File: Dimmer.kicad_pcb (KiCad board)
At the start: 2 copper layers, 63.9 x 63.9 mm, 21 parts, among them IC1 TTP224B-BSBN, J1 Reset, J2 Prog, J3 Conn_01x04, J4 Mode, J5 Load_cntrl, J6 Detect_null, U1 ESP-07, k1 Key, k2 Key, k3 Key

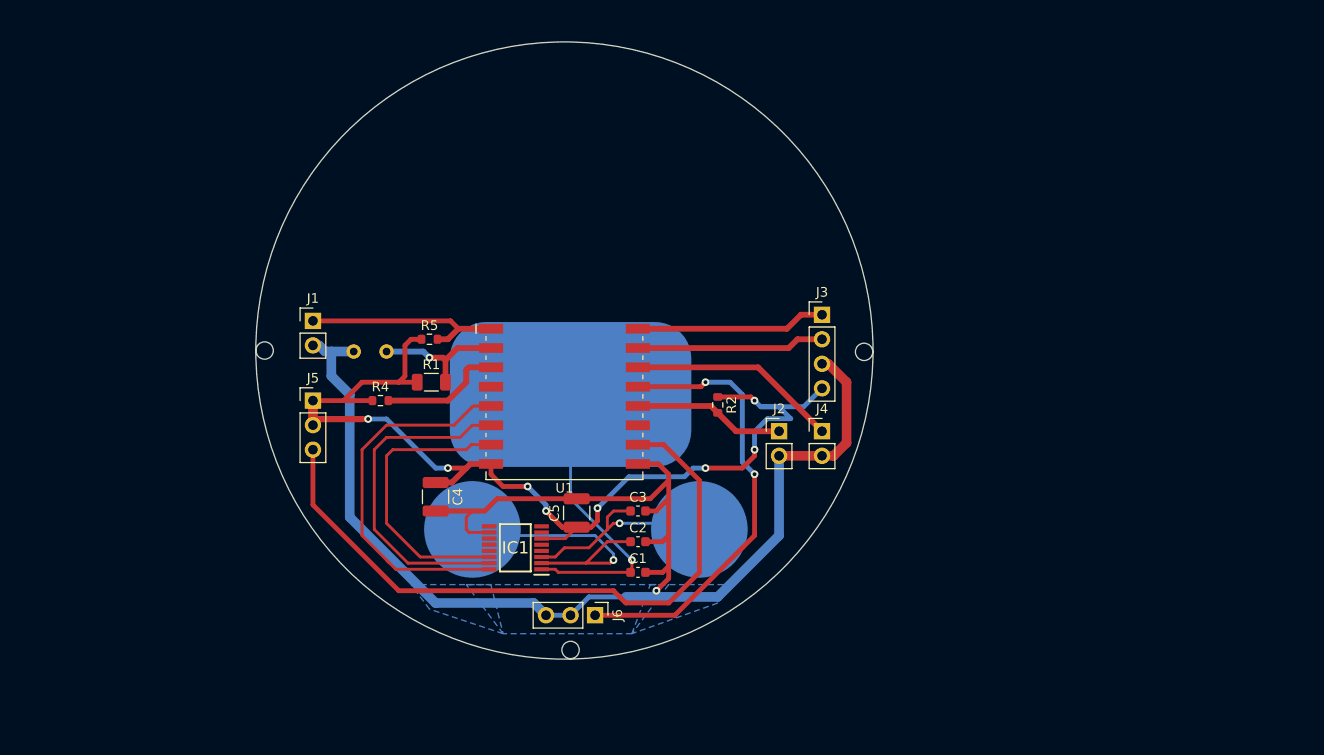
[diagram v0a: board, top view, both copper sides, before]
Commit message: Add files via upload
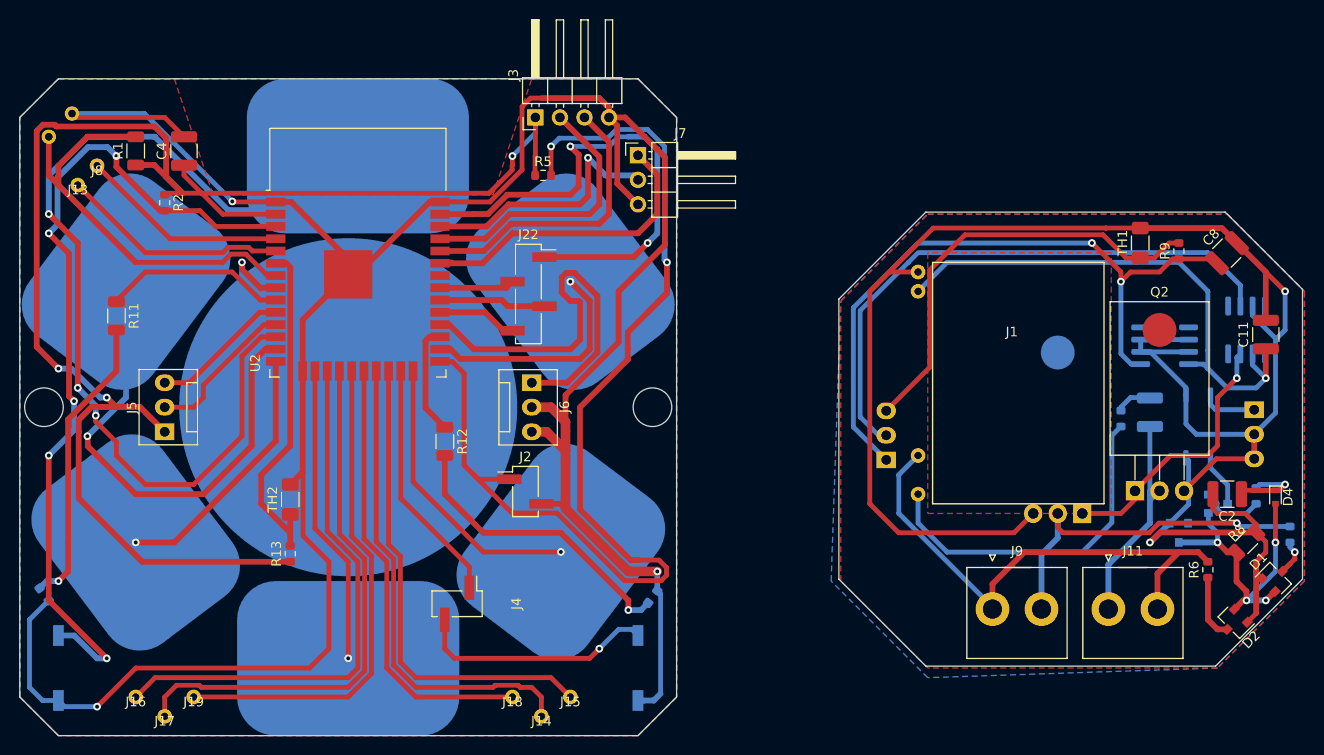
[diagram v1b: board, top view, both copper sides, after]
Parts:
- removed C3: 30p, Capacitor_SMD:C_0603_1608Metric
- removed C5: 100mk, Capacitor_SMD:C_1210_3225Metric
- removed IC1: TTP224B-BSBN, TTP224B-BSBN:SOP64P600X175-16N
- added C11: 0.33mk, Capacitor_SMD:C_1210_3225Metric, F.Cu at (232.0, 100.5)
- added C8: 0.1mk, Capacitor_SMD:C_1210_3225Metric, F.Cu at (228.0, 92.0)
- added D1: BAV99, Package_TO_SOT_SMD:SOT-23, F.Cu at (233.0, 125.7)
- added D2: BAV99, Package_TO_SOT_SMD:SOT-23, F.Cu at (228.7, 130.3)
- added D3: BZX84Cxx, Diode_SMD:D_SOT-23_ANK, B.Cu at (223.0, 121.0)
- added D4: 1N4148WT, Diode_SMD:D_SOD-523, F.Cu at (233.0, 117.3)
- added D5: BLUE, LED_SMD:LED_0603_1608Metric, B.Cu at (105.5, 127.4)
- added D6: RED, LED_SMD:LED_0603_1608Metric, B.Cu at (168.5, 127.6)
- added J10: Detect_nullA, Connector:FanPinHeader_1x03_P2.54mm_Vertical, B.Cu at (230.8, 108.3)
- added J11: 220v_OUT, Touch_pad:220V_1x02_P5.08mm_Horizontal, F.Cu at (215.7, 125.9)
- added J12: Load_cntrlA, Connector:FanPinHeader_1x03_P2.54mm_Vertical, B.Cu at (192.7, 113.5)
- added J13: ADC, Touch_pad:polz_razjem, F.Cu at (109.0, 85.0)
- added J14: Conn_01x01, Touch_pad:polz_razjem, F.Cu at (157.0, 140.0)
- added J15: Conn_01x01, Touch_pad:polz_razjem, F.Cu at (160.0, 138.0)
- added J16: Conn_01x01, Touch_pad:polz_razjem, F.Cu at (115.0, 138.0)
- added J17: Conn_01x01, Touch_pad:polz_razjem, F.Cu at (118.0, 140.0)
- added J18: Conn_01x01, Touch_pad:polz_razjem, F.Cu at (154.0, 138.0)
- added J19: Conn_01x01, Touch_pad:polz_razjem, F.Cu at (121.0, 138.0)
- added J22: SPI, Connector_PinHeader_2.54mm:PinHeader_1x04_P2.54mm_Vertical_SMD_Pin1Right, F.Cu at (155.7, 96.3)
- added J7: I2C, Connector_PinHeader_2.54mm:PinHeader_1x03_P2.54mm_Horizontal, F.Cu at (167.0, 81.9)
- added J8: ADC, Touch_pad:polz_razjem, F.Cu at (111.0, 83.0)
- added J9: 220v_IN, Touch_pad:220V_1x02_P5.08mm_Horizontal, F.Cu at (203.7, 125.9)
- added Q1: IRFP460APBF, Package_TO_SOT_THT:TO-220-3_Horizontal_TabDown, B.Cu at (213.0, 119.0)
- added Q2: IRFP460APBF, Package_TO_SOT_THT:TO-220-3_Horizontal_TabDown, F.Cu at (218.5, 116.7)
- added Q3: BC807, Package_TO_SOT_SMD:SOT-23, B.Cu at (227.1, 118.0)
- added R10: 220, Resistor_SMD:R_0603_1608Metric, B.Cu at (231.0, 117.2)
- added R11: 220, Resistor_SMD:R_1206_3216Metric, F.Cu at (113.0, 98.5)
- added R12: 220, Resistor_SMD:R_1206_3216Metric, F.Cu at (147.0, 111.5)
- added R13: 10k, Resistor_SMD:R_0603_1608Metric, F.Cu at (131.0, 123.2)
- added R6: 120k 0.25W, Resistor_SMD:R_0603_1608Metric, F.Cu at (226.0, 124.8)
- added R7: 220 1W, Resistor_SMD:R_0603_1608Metric, B.Cu at (217.0, 109.2)
- added R8: 330k 0.25W, Resistor_SMD:R_1206_3216Metric, F.Cu at (230.0, 122.0)
- added R9: 10k, Resistor_SMD:R_0603_1608Metric, F.Cu at (223.0, 91.8)
- added SW1: SW_Push, Button_Switch_SMD:SW_DIP_SPSTx01_Slide_6.7x4.1mm_W6.73mm_P2.54mm_LowProfile_JPin, B.Cu at (107.0, 135.0)
- added SW2: SW_Push, Button_Switch_SMD:SW_DIP_SPSTx01_Slide_6.7x4.1mm_W6.73mm_P2.54mm_LowProfile_JPin, B.Cu at (167.0, 135.0)
- added TH1: Thermistor_NTC, Resistor_SMD:R_1206_3216Metric_Pad1.30x1.75mm_HandSolder, F.Cu at (219.0, 91.0)
- added TH2: Thermistor_NTC, Resistor_SMD:R_1206_3216Metric_Pad1.30x1.75mm_HandSolder, F.Cu at (131.0, 117.5)
- added U2: ESP32-WROOM-32D, RF_Module:ESP32-WROOM-32, F.Cu at (138.0, 95.0)
- added U3: L78L33_SO8, Package_SO:SOIC-8_3.9x4.9mm_P1.27mm, B.Cu at (221.5, 101.6)
- added U4: TLP185, Package_SO:SOIC-4_4.55x3.7mm_P2.54mm, B.Cu at (225.0, 110.0)
- added k4: Key, Touch_pad:TestPoint_Pad_1.0x1.0sm, B.Cu at (107.0, 128.0)
- added k5: Key, Touch_pad:TestPoint_Pad_1.0x1.0sm, B.Cu at (137.0, 144.0)
- added k6: Key, Touch_pad:TestPoint_Pad_1.0x1.0sm, B.Cu at (122.0, 101.0)
- added k7: Key, Touch_pad:TestPoint_Pad_1.0x1.0sm, B.Cu at (138.0, 92.0)
- C1: value 30p -> 0.01mk; footprint Capacitor_SMD:C_0603_1608Metric -> Capacitor_SMD:C_1210_3225Metric; moved to B.Cu
- C2: value 30p -> 0.47mk; footprint Capacitor_SMD:C_0603_1608Metric -> Capacitor_SMD:C_1210_3225Metric
- J1: value Reset -> 220to12; footprint Connector_PinHeader_2.54mm:PinHeader_1x02_P2.54mm_Vertical -> Touch_pad:oblast_bp
- J2, J4: footprint Connector_PinHeader_2.54mm:PinHeader_1x02_P2.54mm_Vertical -> Connector_PinHeader_2.54mm:PinHeader_1x02_P2.54mm_Vertical_SMD_Pin1Left
- J3: value Conn_01x04 -> UART0; footprint Connector_PinHeader_2.54mm:PinHeader_1x04_P2.54mm_Vertical -> Connector_PinHeader_2.54mm:PinHeader_1x04_P2.54mm_Horizontal
- J5, J6: footprint Connector_PinHeader_2.54mm:PinHeader_1x03_P2.54mm_Vertical -> Connector:FanPinHeader_1x03_P2.54mm_Vertical
- R4: value 10k -> 120k 0.25W; moved to B.Cu
- U1: value ESP-07 -> FAN3268; footprint RF_Module:ESP-07 -> Package_SO:SOIC-8_3.9x4.9mm_P1.27mm; moved to B.Cu
- k1: footprint Touch_pad:TestPoint_Pad_2.5x2.5sm -> Touch_pad:TestPoint_Pad_1.0x1.0sm
- moved R4 95.2 mm to (234.5, 121.2), turned to 90 degrees
- moved J1 73.4 mm to (206.5, 105.0)
- moved U1 70.8 mm to (230.0, 100.0), turned to 270 degrees
- moved C2 61.2 mm to (228.0, 117.0), turned to 180 degrees
- moved R2 61.0 mm to (118.0, 86.8)
- moved C1 55.5 mm to (220.0, 108.5), turned to 270 degrees
- moved k3 46.4 mm to (137.0, 118.0), turned to 0 degrees
- moved C4 44.3 mm to (120.0, 81.5), turned to 90 degrees
- moved J4 41.8 mm to (148.3, 128.3), turned to 270 degrees
- moved R3 41.4 mm to (106.0, 80.0), turned to 45 degrees
- moved R1 38.9 mm to (115.0, 81.5), turned to 90 degrees
- moved J3 36.0 mm to (156.4, 78.0), turned to 90 degrees
- moved J2 27.0 mm to (155.3, 116.7)
- moved J6 25.0 mm to (156.0, 105.5)
- moved R5 20.6 mm to (157.2, 84.0)
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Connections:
- C1 pad 2: GND -> Net-(C1-Pad2)
- C2 pad 2: GND -> Net-(C2-Pad2)
- J1 pad 2: GND -> +12V
- J3 pad 1: Net-(J3-Pad1) -> +3V3
- J3 pad 3: GND -> Net-(J3-Pad3)
- J3 pad 4: +3V3 -> GND
- J4 pad 1: Net-(J4-Pad1) -> Mode
- J4 pad 2: GND -> Net-(J4-Pad2)
- J5 pad 2: +3V3 -> GPIO26
- J5 pad 3: GPIO15 -> GPIO32
- J6 pad 1: GPIO4 -> GPIO17
- R1 pad 2: Net-(R1-Pad2) -> GPIO35
- R2 pad 2: Net-(J2-Pad1) -> Net-(R2-Pad2)
- R3 pad 1: Net-(R1-Pad2) -> GPIO35
- R4 pad 1: +3V3 -> Net-(D1-Pad3)
- R4 pad 2: Net-(R4-Pad2) -> Net-(J1-Pad1)
- R5 pad 2: Net-(J1-Pad1) -> Net-(J2-Pad1)
- U1 pad 1: Net-(J1-Pad1) -> Net-(U1-Pad1)
- U1 pad 2: Net-(R1-Pad2) -> cntrl
- U1 pad 3: Net-(R4-Pad2) -> GND
- U1 pad 6: Net-(IC1-Pad15) -> +12V
- U1 pad 8: +3V3 -> Net-(U1-Pad8)
- k1 pad 1: Net-(C1-Pad1) -> Net-(U2-Pad26)
- k2 pad 1: Net-(C2-Pad1) -> Net-(U2-Pad24)
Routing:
- net GND: track 159.2 -> 437.4 mm, vias 1 -> 4
- net +3V3: track 115.3 -> 248.5 mm, vias 8 -> 5
- net Net-(U2-Pad12): track 0.00 -> 99.9 mm, vias 0 -> 3
- net Net-(J2-Pad1): track 15.7 -> 115.1 mm, vias 0 -> 2
- net Net-(R2-Pad2): track 0.00 -> 88.7 mm, vias 0 -> 5
- net GPIO15: track 68.7 -> 0.00 mm
- net cntrl: track 0.00 -> 59.7 mm
- net Net-(J16-Pad1): track 0.00 -> 56.3 mm
- net Net-(J17-Pad1): track 0.00 -> 56.1 mm
- net +12V: track 0.00 -> 56.1 mm, vias 0 -> 1
- net Net-(J1-Pad3): track 0.00 -> 54.2 mm
- net Net-(J19-Pad1): track 0.00 -> 51.6 mm
- net Net-(U2-Pad13): track 0.00 -> 51.5 mm, vias 0 -> 1
- net MOSI: track 0.00 -> 51.4 mm, vias 0 -> 2
- net Net-(J1-Pad1): track 21.4 -> 72.8 mm, vias 0 -> 1
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- added copper zone on F.Cu, net GND
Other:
- board size 63.9 x 63.9 mm -> 132.8 x 68 mm
- net class Default: trace_width 0.6 -> 0.25
- rule trace_min: 0.3 -> 0.2
- rule via_min_drill: 0.2 -> 0.3
- rule via_min_size: 0.3 -> 0.4
